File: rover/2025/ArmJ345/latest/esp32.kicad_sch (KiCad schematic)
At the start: 15 parts, among them SW1 SW-PTS815SJM250SMTRLFS, SW2 SW-PTS815SJM250SMTRLFS, U7 ESP32-S3-WROVER

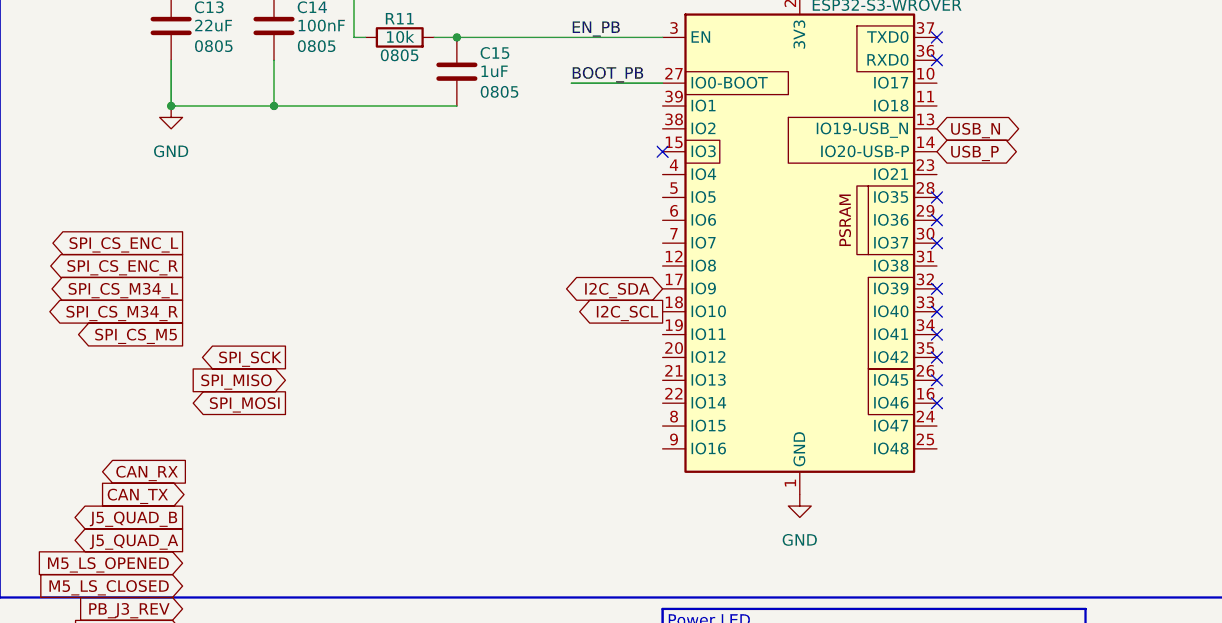
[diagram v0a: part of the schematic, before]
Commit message: .
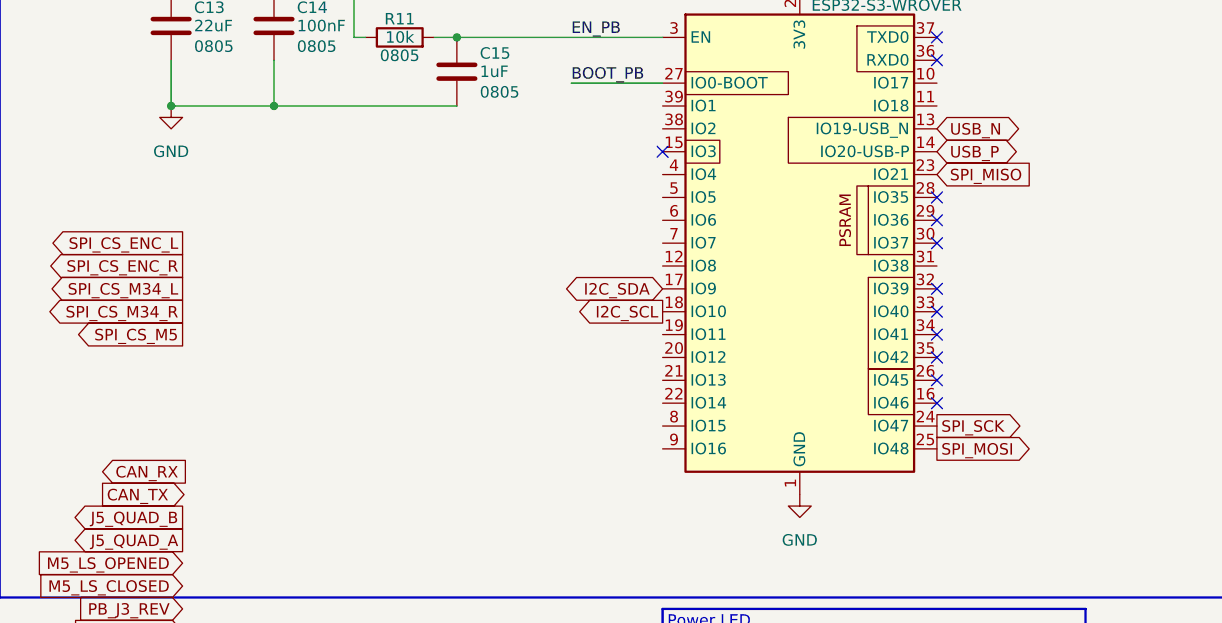
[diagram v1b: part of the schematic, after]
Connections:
- net SPI_MISO: now also U7.23 (IO21)
- net SPI_MOSI: now also U7.25 (IO48)
- net SPI_SCK: now also U7.24 (IO47)
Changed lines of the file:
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@@
 	(global_label "SPI_MOSI"
 		(shape output)
-		(at 44.45 72.39 180)
+		(at 116.84 77.47 0)
 		(fields_autoplaced yes)
 		(effects
@@
 				(size 1.27 1.27)
 			)
-			(justify right)
+			(justify left)
 		)
 		(property "Intersheetrefs" "${INTERSHEET_REFS}"
-			(at 32.8167 72.39 0)
+			(at 128.4733 77.47 0)
 			(effects
 				(font
 					(size 1.27 1.27)
 				)
-				(justify right)
+				(justify left)
 				(hide yes)
 			)
@@
 	(global_label "SPI_MISO"
 		(shape input)
-		(at 44.45 69.85 180)
+		(at 116.84 46.99 0)
 		(fields_autoplaced yes)
 		(effects
@@
 				(size 1.27 1.27)
 			)
-			(justify right)
+			(justify left)
 		)
 		(property "Intersheetrefs" "${INTERSHEET_REFS}"
-			(at 32.8167 69.85 0)
+			(at 128.4733 46.99 0)
 			(effects
 				(font
 					(size 1.27 1.27)
 				)
-				(justify right)
+				(justify left)
 				(hide yes)
 			)
@@
 	(global_label "SPI_SCK"
 		(shape output)
-		(at 44.45 67.31 180)
+		(at 116.84 74.93 0)
 		(fields_autoplaced yes)
 		(effects
@@
 				(size 1.27 1.27)
 			)
-			(justify right)
+			(justify left)
 		)
 		(property "Intersheetrefs" "${INTERSHEET_REFS}"
-			(at 33.6634 67.31 0)
+			(at 127.6266 74.93 0)
 			(effects
 				(font
 					(size 1.27 1.27)
 				)
-				(justify right)
+				(justify left)
 				(hide yes)
 			)

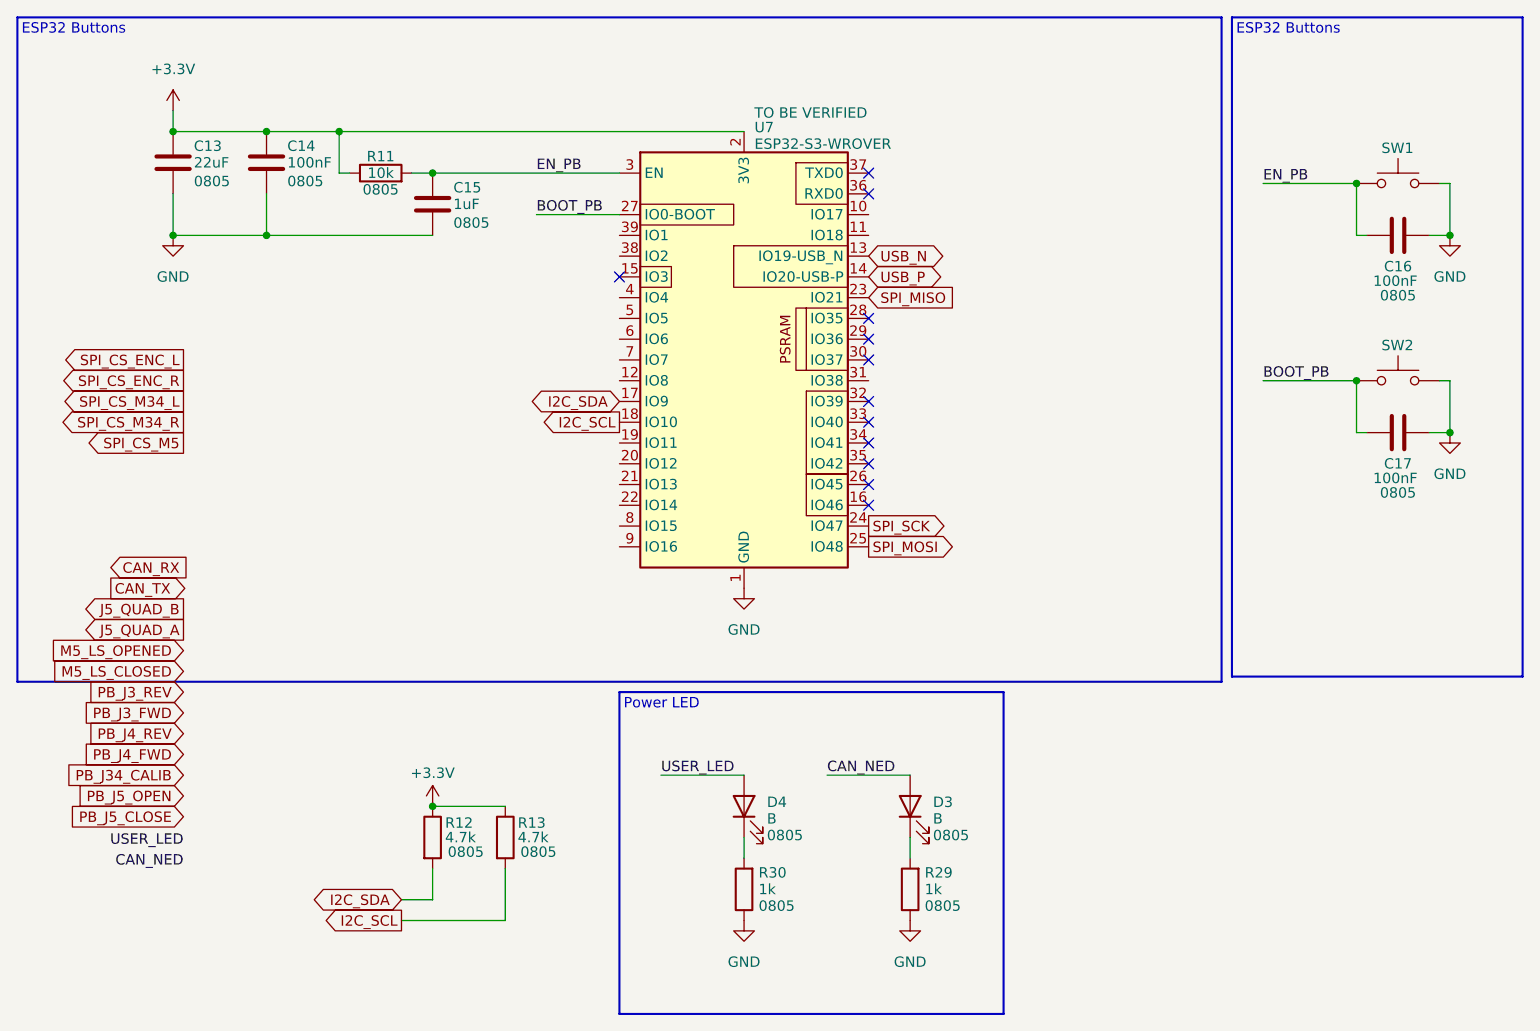
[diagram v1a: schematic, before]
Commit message: ARMJ345 V0 done
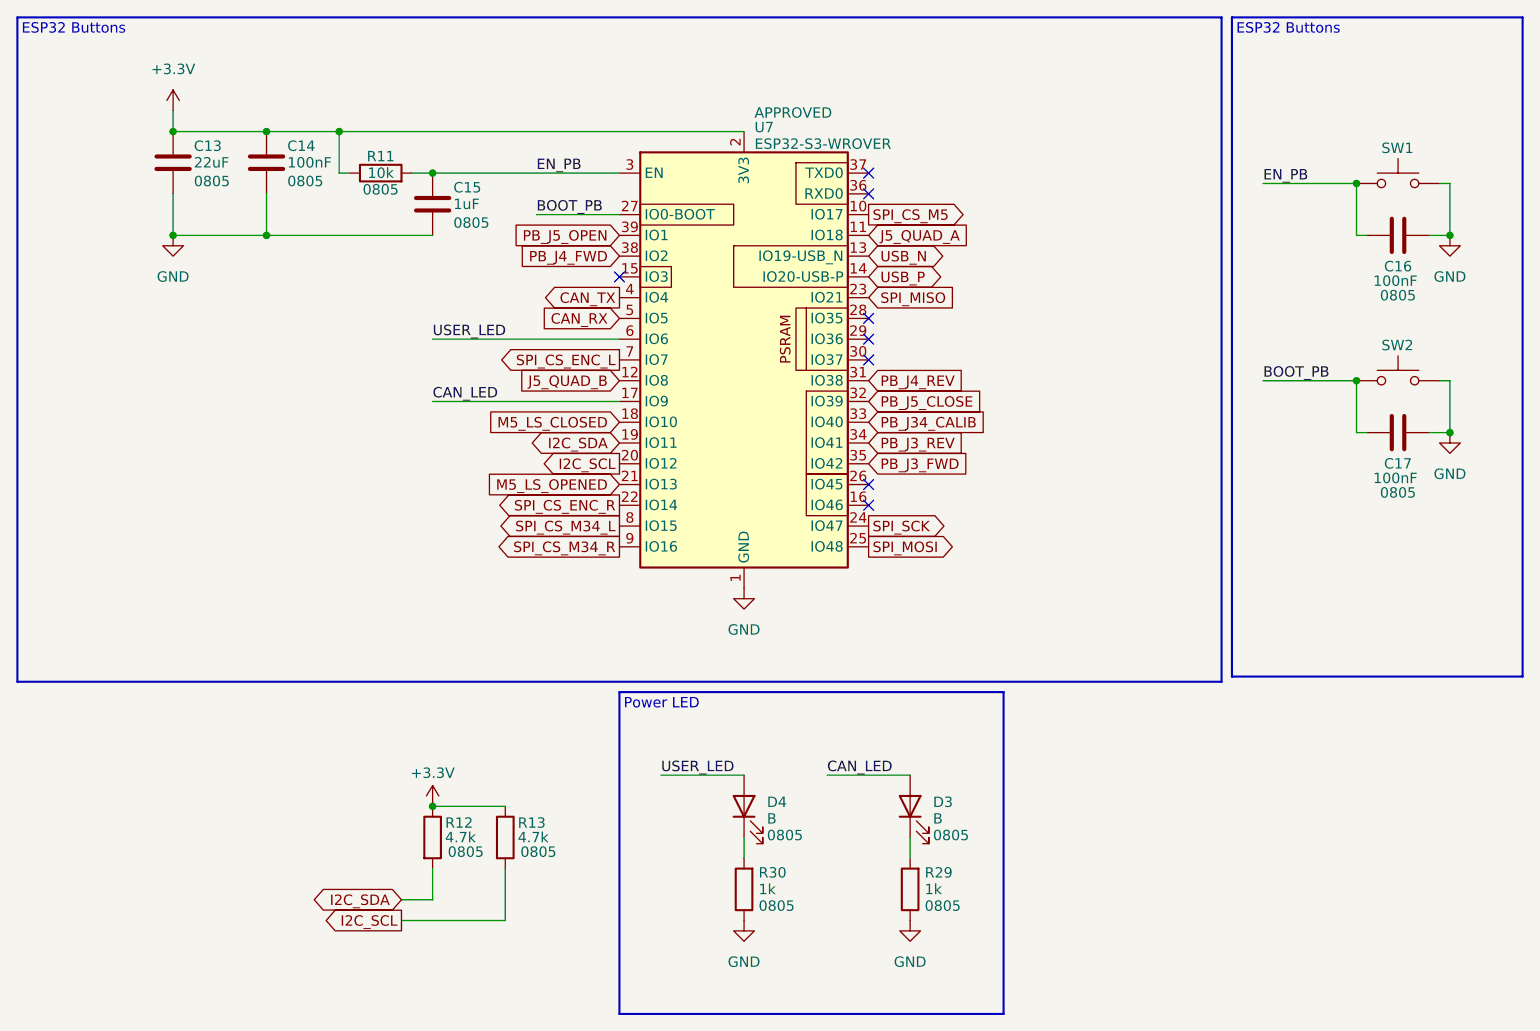
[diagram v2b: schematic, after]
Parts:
- U7: STATUS TO BE VERIFIED -> APPROVED
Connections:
- net CAN_RX: now also U7.5 (IO5)
- net CAN_TX: now also U7.4 (IO4)
- net I2C_SCL: now also U7.20 (IO12); no longer U7.18 (IO10)
- net I2C_SDA: now also U7.19 (IO11); no longer U7.17 (IO9)
- net J5_QUAD_A: now also U7.11 (IO18)
- net J5_QUAD_B: now also U7.12 (IO8)
- net M5_LS_CLOSED: now also U7.18 (IO10)
- net M5_LS_OPENED: now also U7.21 (IO13)
- net PB_J34_CALIB: now also U7.33 (IO40)
- net PB_J3_FWD: now also U7.35 (IO42)
- net PB_J3_REV: now also U7.34 (IO41)
- net PB_J4_FWD: now also U7.38 (IO2)
- net PB_J4_REV: now also U7.31 (IO38)
- net PB_J5_CLOSE: now also U7.32 (IO39)
- net PB_J5_OPEN: now also U7.39 (IO1)
- net SPI_CS_ENC_L: now also U7.7 (IO7)
- net SPI_CS_ENC_R: now also U7.22 (IO14)
- net SPI_CS_M34_L: now also U7.8 (IO15)
- net SPI_CS_M34_R: now also U7.9 (IO16)
- net SPI_CS_M5: now also U7.10 (IO17)
- net USER_LED: now also U7.6 (IO6)
- net CAN_NED renamed CAN_LED
- net CAN_LED: now also U7.17 (IO9)
- no-connect marks 12 -> 8
